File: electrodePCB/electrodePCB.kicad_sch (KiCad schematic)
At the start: 21 parts, among them J1 Conn_01x20, U1 TMP119AIYBGR

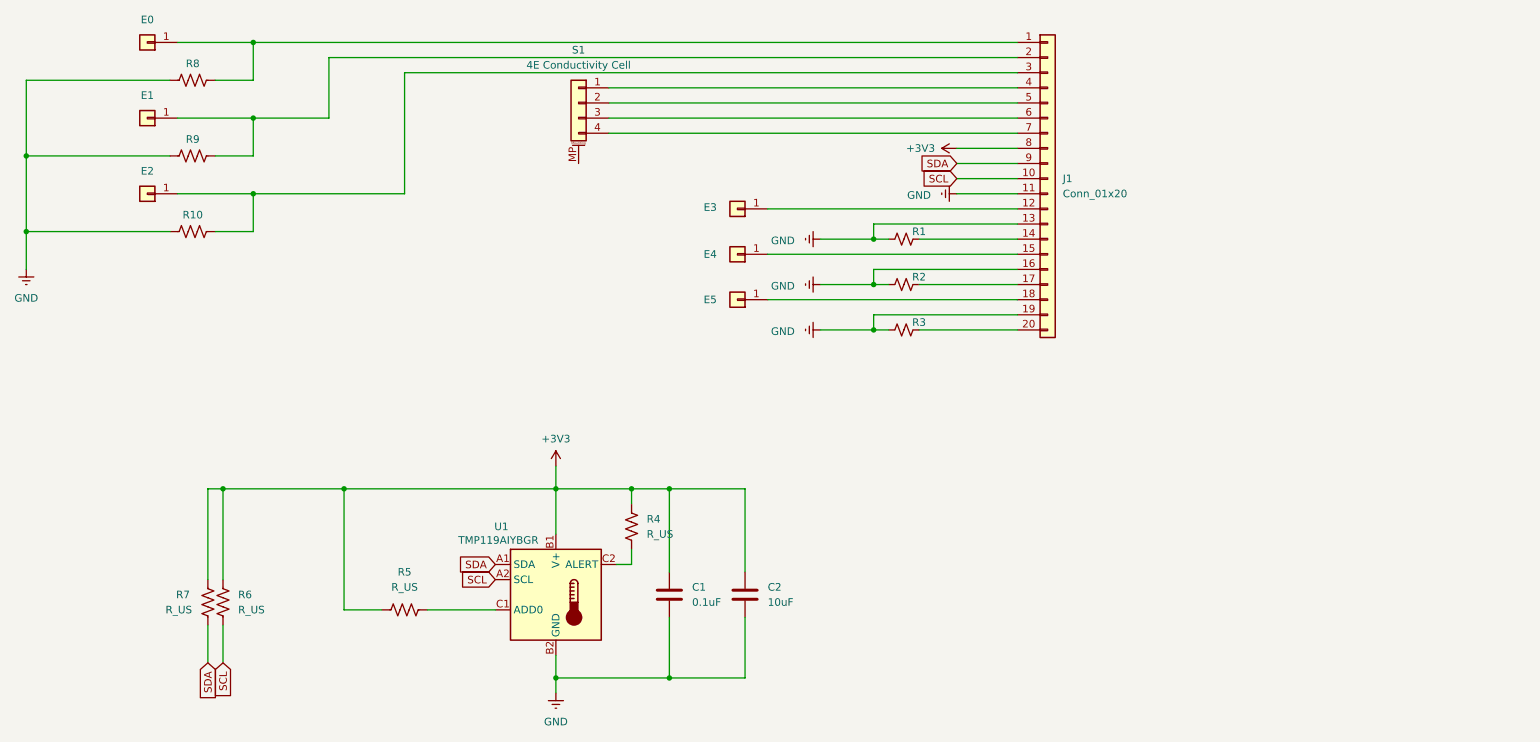
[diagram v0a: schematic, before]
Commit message: routing, routing, routing. We removed one of the three heaters and decided to displace the other two and route to rings around the electrodes. I verified the temperature sensor is work!
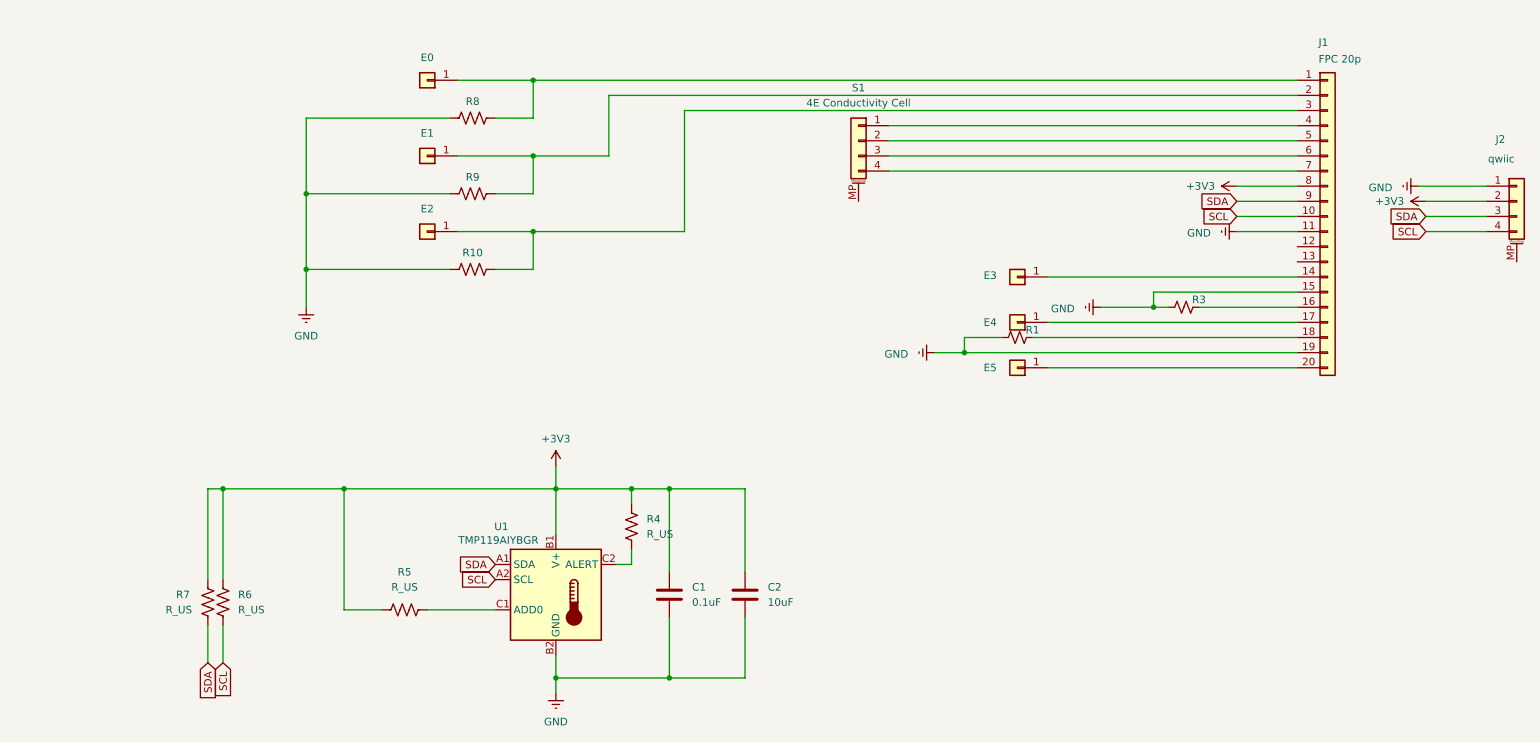
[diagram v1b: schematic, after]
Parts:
- removed R2: R_Small_US, Resistor_SMD:adjustable, symbol Device:R_Small_US
- added J2: qwiic, Connector_JST:JST_SH_BM04B-SRSS-TB_1x04-1MP_P1.00mm_Vertical, symbol Connector_Generic_MountingPin:Conn_01x04_MountingPin
- J1: value Conn_01x20 -> FPC 20p
- R1, R3: footprint Resistor_SMD:R_2512_6332Metric_Pad1.40x3.35mm_HandSolder -> Resistor_SMD:R_2010_5025Metric
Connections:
- net +3V3: now also J2.2 (Pin_2)
- net GND: now also J1.15 (Pin_15), J2.1 (Pin_1); no longer J1.13 (Pin_13), J1.16 (Pin_16)
- net SCL: now also J2.4 (Pin_4)
- net SDA: now also J2.3 (Pin_3)
- net at E3.1 (Pin_1): now also J1.14 (Pin_14); no longer J1.12 (Pin_12)
- net at R1.1: now also J1.18 (Pin_18); no longer J1.14 (Pin_14)
- net at E4.1 (Pin_1): now also J1.17 (Pin_17); no longer J1.15 (Pin_15)
- net at R3.1: now also J1.16 (Pin_16); no longer J1.20 (Pin_20)
- net at E5.1 (Pin_1): now also J1.20 (Pin_20); no longer J1.18 (Pin_18)
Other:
- moved on the sheet: E0, E1, E2, E3, E4, E5, J1, R1, R10, R3, R8, R9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
